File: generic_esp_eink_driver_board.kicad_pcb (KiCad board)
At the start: 2 copper layers, 160 x 25 mm, 53 parts, among them IC1 TPS7A0233PDBVR, IC2 MAX17260SETD+T, J1 USB_C_Receptacle_USB2.0_16P, J2 S2B-PH-SM4-TB, J3 Conn_01x04, Q1 AO3400A, U1 USBLC6-2SC6, U2 BQ24040DSQR, U3 ESP32-S3-WROOM-1, U4 FPC24

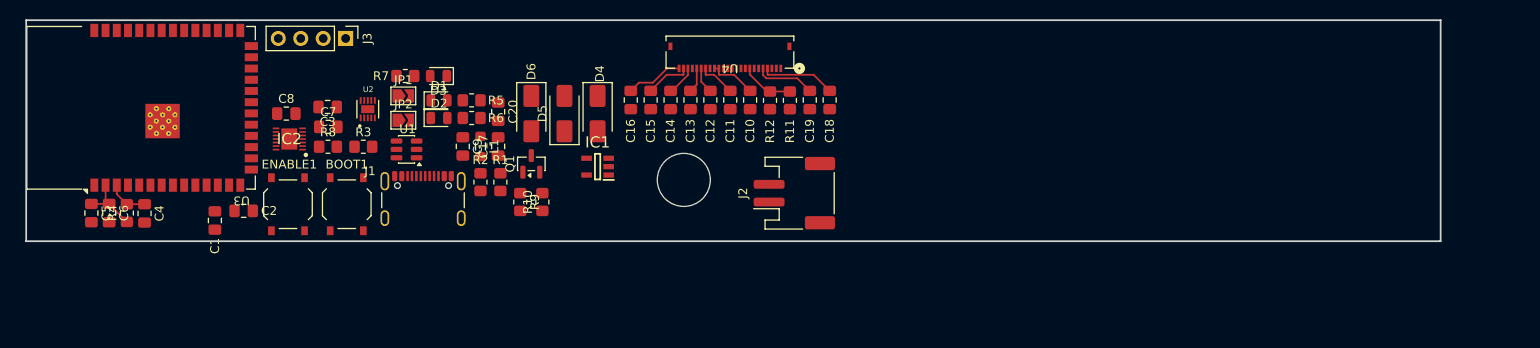
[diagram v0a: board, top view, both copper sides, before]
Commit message: re-placement
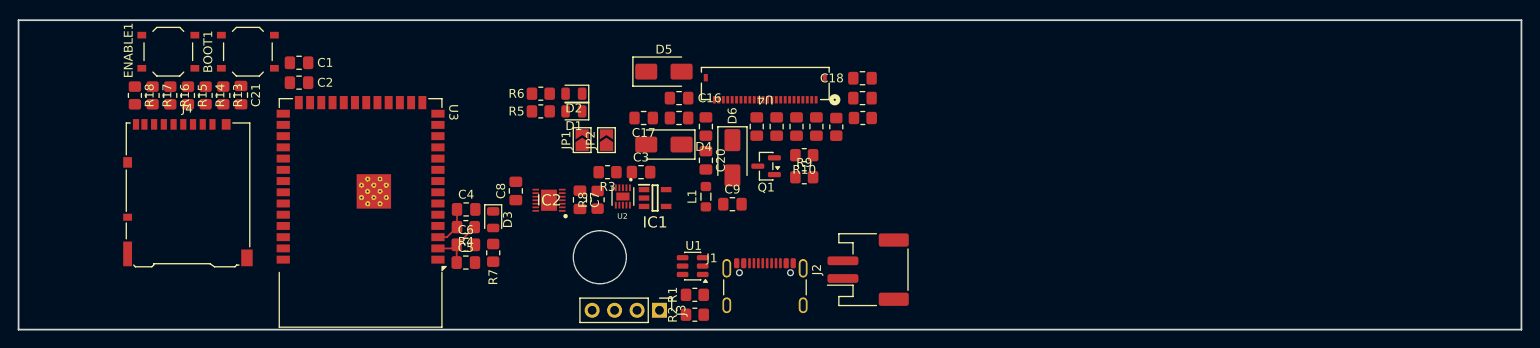
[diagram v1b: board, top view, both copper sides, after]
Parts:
- added C21: 100nF, Capacitor_SMD:C_0805_2012Metric_Pad1.18x1.45mm_HandSolder, F.Cu at (70.2, 73.2)
- added J4: Micro_SD_Card_Det_Hirose_DM3AT, Connector_Card:microSD_HC_Hirose_DM3AT-SF-PEJM5, F.Cu at (64.2, 84.2)
- added R13: 10k, Resistor_SMD:R_0805_2012Metric_Pad1.20x1.40mm_HandSolder, F.Cu at (68.2, 73.2)
- added R14: 10k, Resistor_SMD:R_0805_2012Metric_Pad1.20x1.40mm_HandSolder, F.Cu at (66.2, 73.2)
- added R15: 10k, Resistor_SMD:R_0805_2012Metric_Pad1.20x1.40mm_HandSolder, F.Cu at (64.2, 73.2)
- added R16: 10k, Resistor_SMD:R_0805_2012Metric_Pad1.20x1.40mm_HandSolder, F.Cu at (62.2, 73.2)
- added R17: 10k, Resistor_SMD:R_0805_2012Metric_Pad1.20x1.40mm_HandSolder, F.Cu at (60.2, 73.2)
- added R18: 10k, Resistor_SMD:R_0805_2012Metric_Pad1.20x1.40mm_HandSolder, F.Cu at (58.2, 73.2)
- moved J3 47.0 mm to (117.5, 97.5)
- moved C5 42.7 mm to (95.6, 92.1), turned to 0 degrees
- moved C6 40.5 mm to (95.6, 90.1), turned to 0 degrees
- moved J1 39.9 mm to (129.4, 95.9)
- moved R4 38.4 mm to (95.6, 88.1), turned to 180 degrees
- moved C4 36.4 mm to (95.6, 86.1), turned to 0 degrees
- moved C3 36.2 mm to (115.4, 81.9), turned to 0 degrees
- moved U1 35.0 mm to (121.2, 92.5)
- moved R9 32.2 mm to (133.9, 82.5), turned to 0 degrees
- moved C9 31.2 mm to (125.8, 85.5), turned to 0 degrees
- moved R8 31.1 mm to (110.5, 85.0), turned to 90 degrees
- moved U2 30.5 mm to (113.4, 84.6), turned to -90 degrees
- moved IC2 30.2 mm to (105.0, 85.0)
- moved R10 30.1 mm to (133.9, 80.0), turned to 180 degrees
- moved C7 29.6 mm to (108.5, 85.0), turned to -90 degrees
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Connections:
- R7 pad 1: Net-(U3-IO39) -> Net-(U3-IO4)
- U3 pad 24: unconnected-(U3-IO47-Pad24) -> SD_D1
- U3 pad 25: unconnected-(U3-IO48-Pad25) -> SD_DET
- U3 pad 31: unconnected-(U3-IO38-Pad31) -> SD_D2
- U3 pad 32: Net-(U3-IO39) -> SD_D3
- U3 pad 33: unconnected-(U3-IO40-Pad33) -> SD_CMD
- U3 pad 34: unconnected-(U3-IO41-Pad34) -> SD_CLK
- U3 pad 35: unconnected-(U3-IO42-Pad35) -> SD_D0
- U3 pad 4: unconnected-(U3-IO4-Pad4) -> Net-(U3-IO4)
- U3 pad 8: FG_SDA -> FG_SCL
- U3 pad 9: FG_SCL -> FG_SDA
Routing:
- net Net-(C18-Pad2): track 8.48 -> 0.00 mm
- net Net-(C19-Pad2): track 6.77 -> 0.00 mm
- net Net-(D5-A): track 6.52 -> 0.00 mm
- net Net-(R11-Pad2): track 6.02 -> 0.00 mm
- net 3V3: track 12.6 -> 7.16 mm
- net Net-(C15-Pad2): track 5.17 -> 0.00 mm
- net Net-(C11-Pad2): track 4.23 -> 0.00 mm
- net Net-(C14-Pad2): track 3.46 -> 0.00 mm
- net Net-(C12-Pad2): track 2.96 -> 0.00 mm
- net Net-(C13-Pad2): track 2.83 -> 0.00 mm
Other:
- board size 160 x 25 mm -> 170 x 35 mm
- board text added: "Battery"
